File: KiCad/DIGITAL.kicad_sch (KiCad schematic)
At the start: 28 parts, among them J7 DE9_Socket, J8 DE9_Pins, SW10 SW_Push, SW11 SW_Push, SW12 SW_Push, SW13 SW_Push, SW14 SW_Push, SW15 SW_Push, SW9 SW_Push, U11 MAX3232, U3 MCP2562-E-SN, U6 24LC256

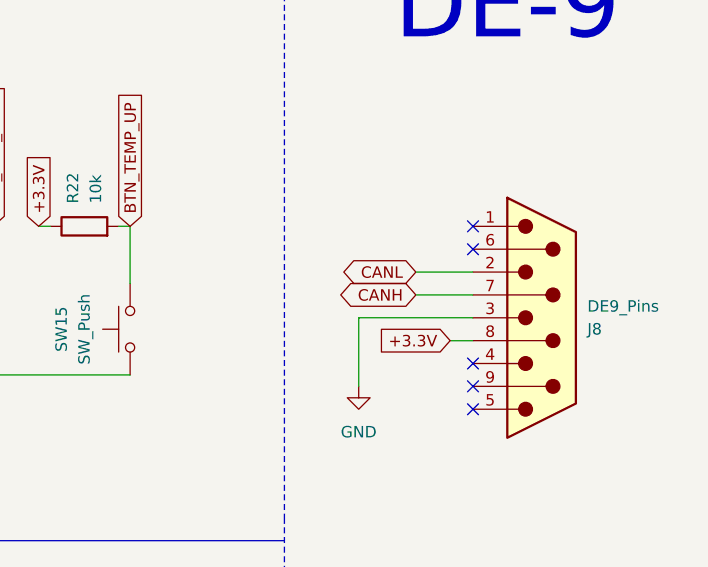
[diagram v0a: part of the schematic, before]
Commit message: ROUTING FINAL
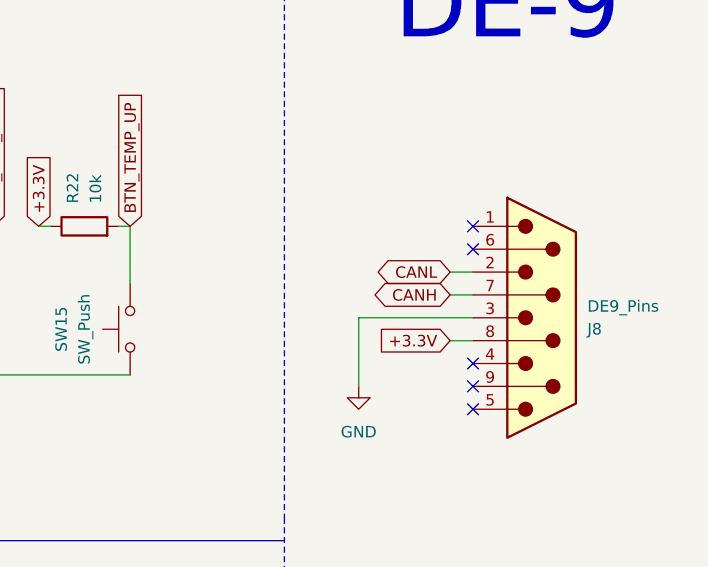
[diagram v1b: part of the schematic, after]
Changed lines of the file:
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@@
 	(wire
 		(pts
-			(xy 252.73 63.5) (xy 259.08 63.5)
+			(xy 256.54 63.5) (xy 259.08 63.5)
 		)
 		(stroke
@@
 	(wire
 		(pts
-			(xy 252.73 60.96) (xy 259.08 60.96)
+			(xy 256.54 60.96) (xy 259.08 60.96)
 		)
 		(stroke
@@
 	(global_label "CANL"
 		(shape bidirectional)
-		(at 252.73 60.96 180)
+		(at 256.54 60.96 180)
 		(fields_autoplaced yes)
 		(effects
@@
 		)
 		(property "Intersheetrefs" "${INTERSHEET_REFS}"
-			(at 243.9163 60.96 0)
+			(at 247.7263 60.96 0)
 			(effects
 				(font
@@
 	(global_label "CANH"
 		(shape bidirectional)
-		(at 252.73 63.5 180)
+		(at 256.54 63.5 180)
 		(fields_autoplaced yes)
 		(effects
@@
 		)
 		(property "Intersheetrefs" "${INTERSHEET_REFS}"
-			(at 243.6139 63.5 0)
-			(effects
-				(font
+			(at 247.4239 63.5 0)
+			(effects
+				(font
